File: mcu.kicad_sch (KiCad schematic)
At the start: 33 parts, among them J1 U.FL-R-SMT-1(10), U1 SF32LB525UC6, U2 MKDV1GCL-ABF, Y1 48MHz, Y2 32.768khz

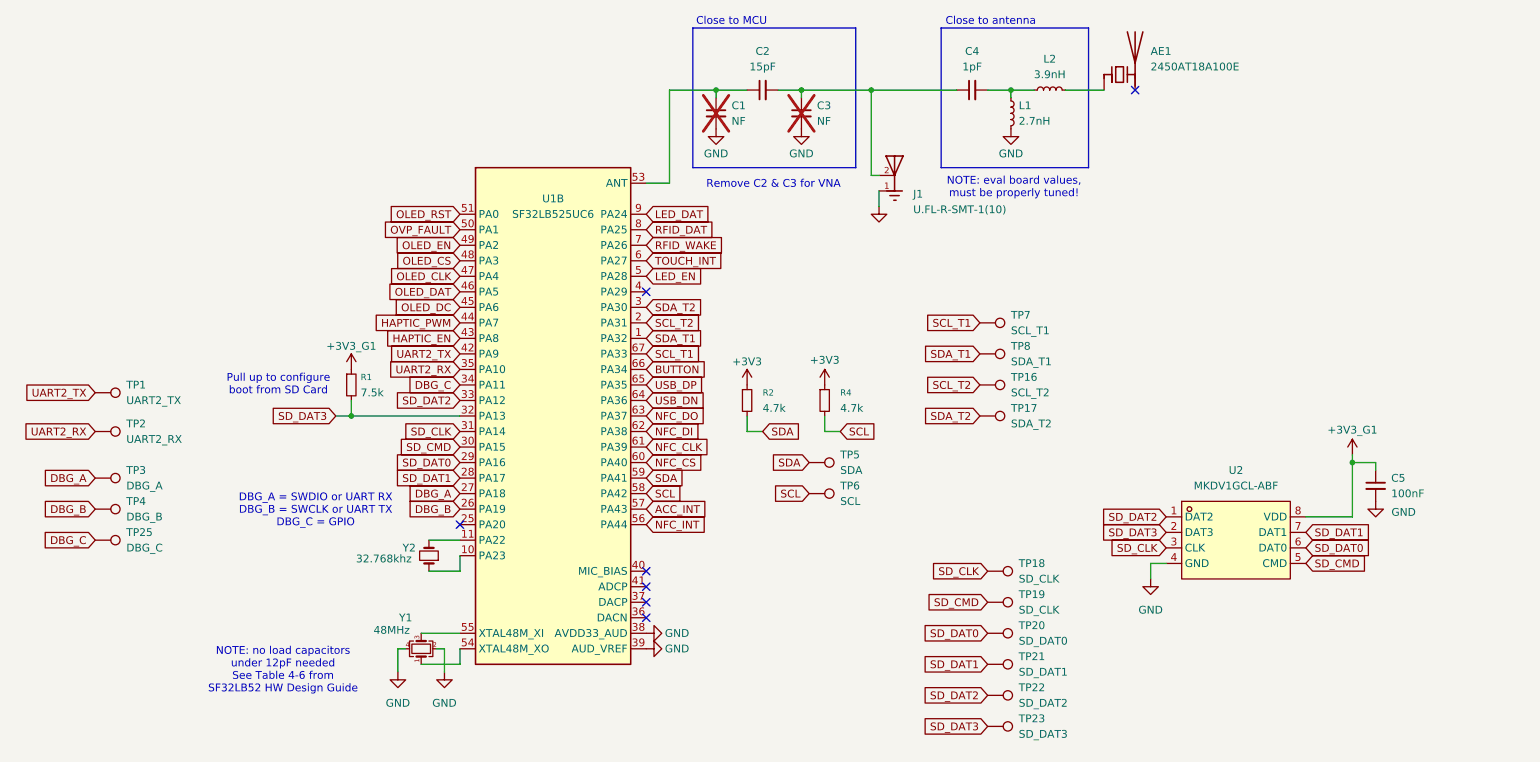
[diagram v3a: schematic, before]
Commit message: fixups before manufacturing pt2
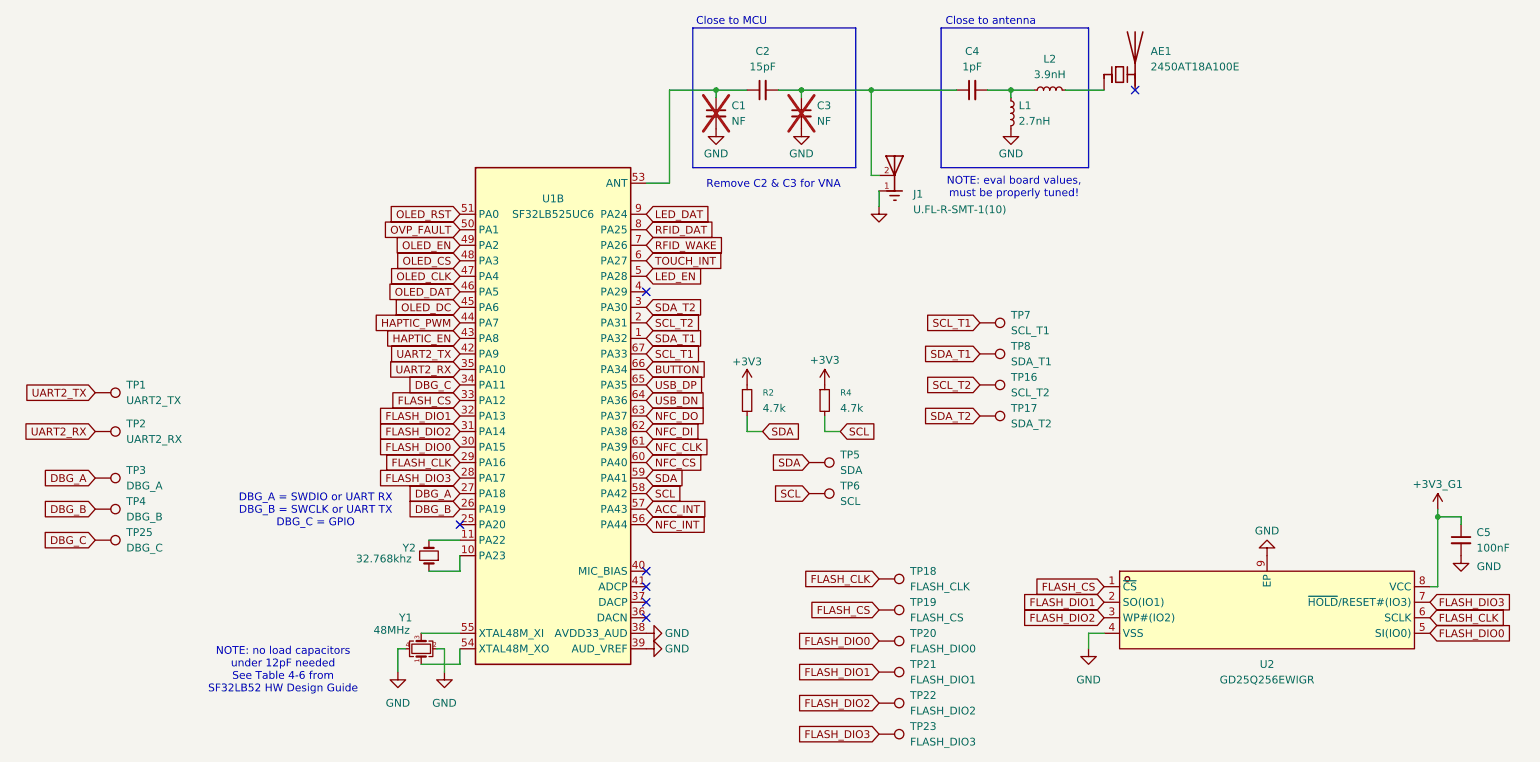
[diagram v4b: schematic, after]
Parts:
- removed R1: 7.5k, Resistor_SMD:R_0603_1608Metric, symbol Device:R_Small
- removed U2: MKDV1GCL-ABF, MKDV1GCL-ABA:LGA-8_L6.0-W8.0-P1.27-TL, symbol MKDV1GCL-ABA:MKDV1GCL-ABA
- added U2: GD25Q256EWIGR, GD25Q256EWIGR:WSON-8_L6.0-W5.0-P1.27-TL-EP, symbol GD25Q256EWIGR:GD25Q256EWIGR
- TP18: value SD_CLK -> FLASH_CLK
- TP19: value SD_CLK -> FLASH_CS
- TP20: value SD_DAT0 -> FLASH_DIO0
- TP21: value SD_DAT1 -> FLASH_DIO1
- TP22: value SD_DAT2 -> FLASH_DIO2
- TP23: value SD_DAT3 -> FLASH_DIO3
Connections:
- net +3V3_G1: now also U2.8 (VCC)
- net GND: now also U2.4 (VSS), U2.9 (EP)
- net SD_CLK renamed FLASH_CLK
- net FLASH_CLK: now also U1.29 (PA16), U2.6 (SCLK); no longer U1.31 (PA14)
- net SD_CMD renamed FLASH_CS
- net FLASH_CS: now also U1.33 (PA12), U2.1 (~{CS}); no longer U1.30 (PA15)
- net SD_DAT0 renamed FLASH_DIO0
- net FLASH_DIO0: now also U1.30 (PA15), U2.5 (SI(IO0)); no longer U1.29 (PA16)
- net SD_DAT1 renamed FLASH_DIO1
- net FLASH_DIO1: now also U1.32 (PA13), U2.2 (SO(IO1)); no longer U1.28 (PA17)
- net SD_DAT2 renamed FLASH_DIO2
- net FLASH_DIO2: now also U1.31 (PA14), U2.3 (WP#(IO2)); no longer U1.33 (PA12)
- net SD_DAT3 renamed FLASH_DIO3
- net FLASH_DIO3: now also U1.28 (PA17), U2.7 (~{HOLD}/RESET#(IO3)); no longer U1.32 (PA13)
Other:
- note removed: "Pull up to configure boot from SD Card"
- moved on the sheet: C5, TP18, TP19, TP20, TP21, TP22, TP23

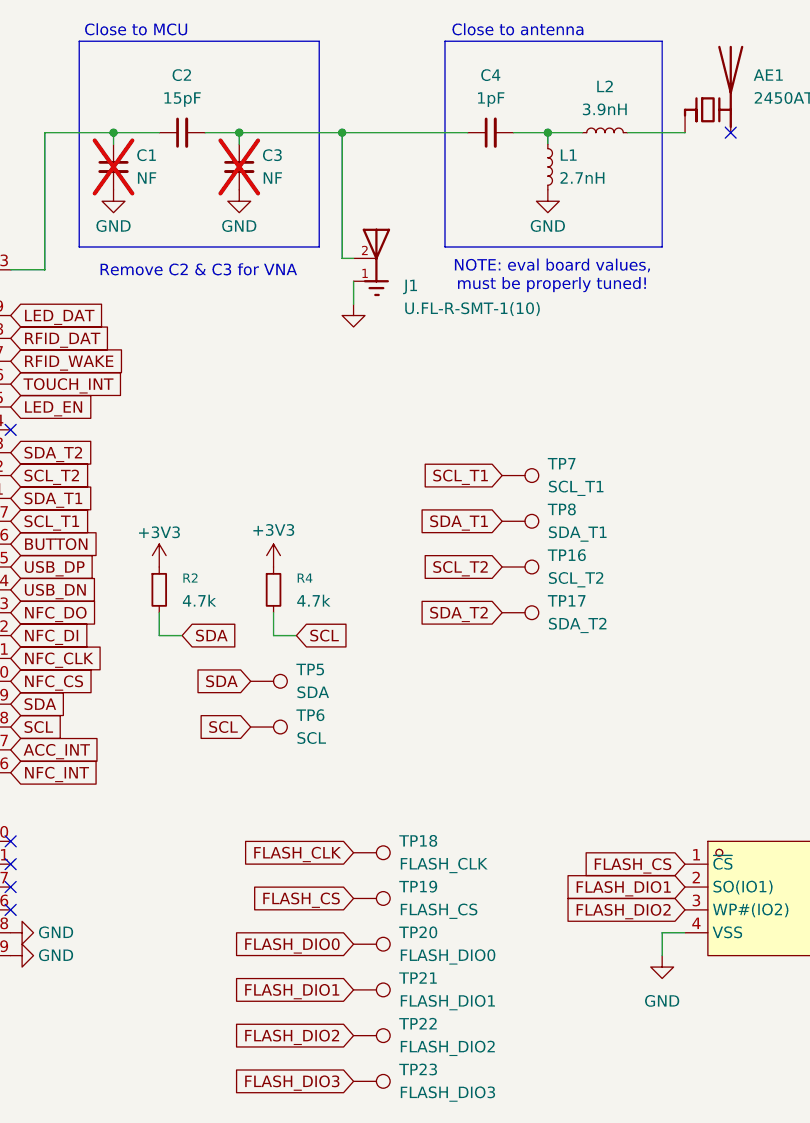
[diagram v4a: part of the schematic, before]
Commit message: layout progress
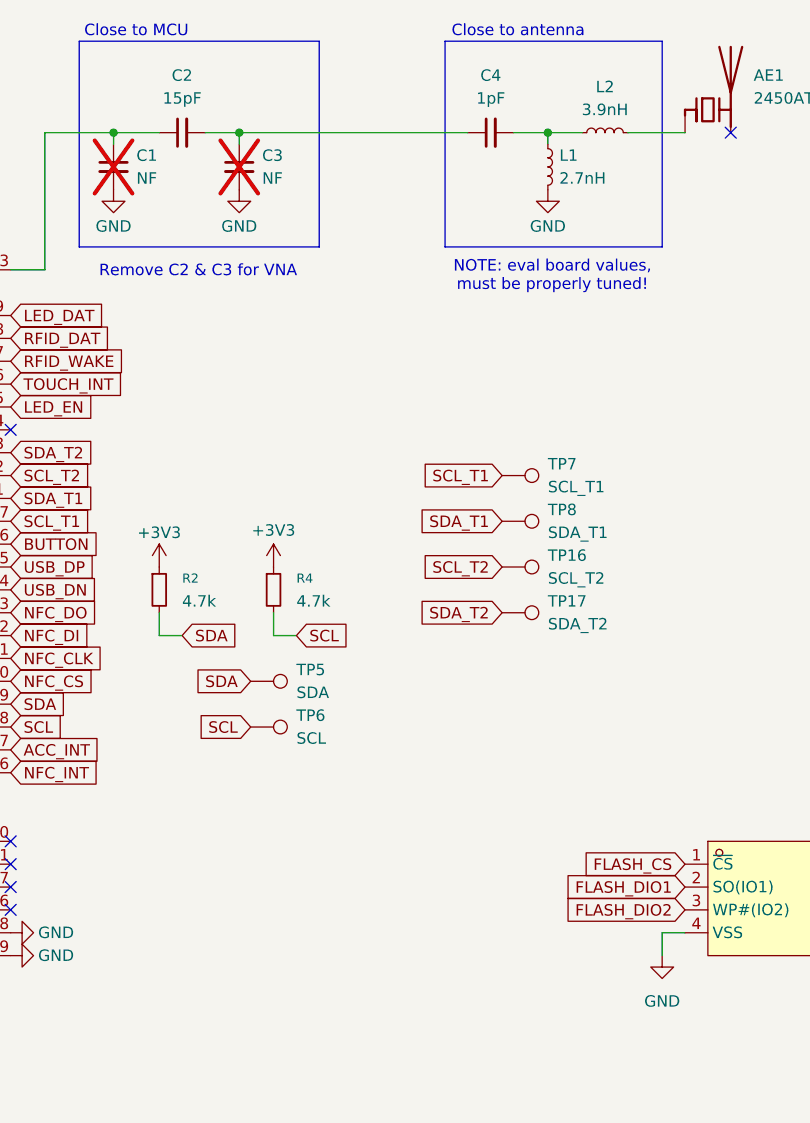
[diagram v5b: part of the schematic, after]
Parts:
- removed J1: U.FL-R-SMT-1(10), U.FL-R-SMT-1_10_:HRS_U.FL-R-SMT-1_10_, symbol U.FL-R-SMT-1_10_:U.FL-R-SMT-1_10_
- removed TP18: FLASH_CLK, TestPoint:TestPoint_Pad_D1.0mm, symbol Connector:TestPoint
- removed TP19: FLASH_CS, TestPoint:TestPoint_Pad_D1.0mm, symbol Connector:TestPoint
- removed TP20: FLASH_DIO0, TestPoint:TestPoint_Pad_D1.0mm, symbol Connector:TestPoint
- removed TP21: FLASH_DIO1, TestPoint:TestPoint_Pad_D1.0mm, symbol Connector:TestPoint
- removed TP22: FLASH_DIO2, TestPoint:TestPoint_Pad_D1.0mm, symbol Connector:TestPoint
- removed TP23: FLASH_DIO3, TestPoint:TestPoint_Pad_D1.0mm, symbol Connector:TestPoint

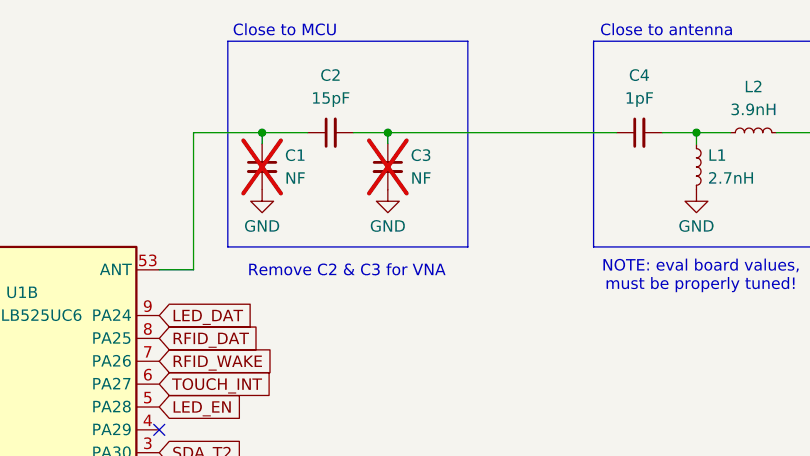
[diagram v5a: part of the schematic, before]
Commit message: progress
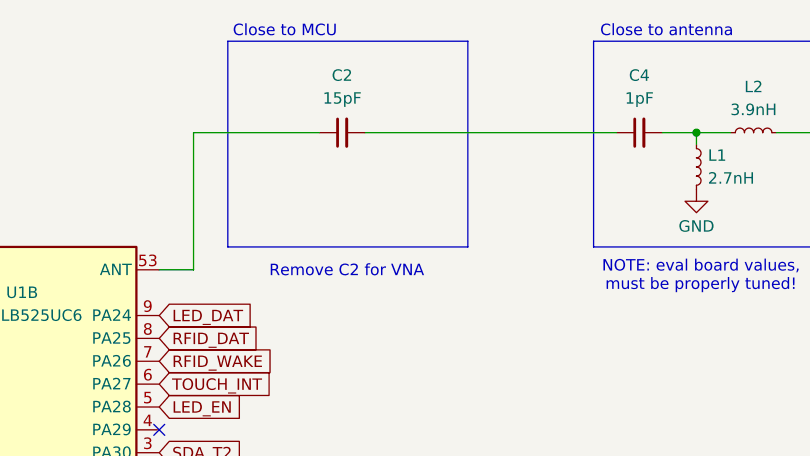
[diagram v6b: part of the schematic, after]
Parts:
- removed C1, C3: NF, Capacitor_SMD:C_0402_1005Metric, symbol Device:C_Small
- Y1: footprint Crystal:Crystal_SMD_2520-4Pin_2.5x2.0mm -> Crystal:Crystal_SMD_2016-4Pin_2.0x1.6mm; LCSC Part C2932991 -> C49363531
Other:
- note added: "Remove C2 for VNA"
- note removed: "Remove C2 & C3 for VNA"
- moved on the sheet: C2

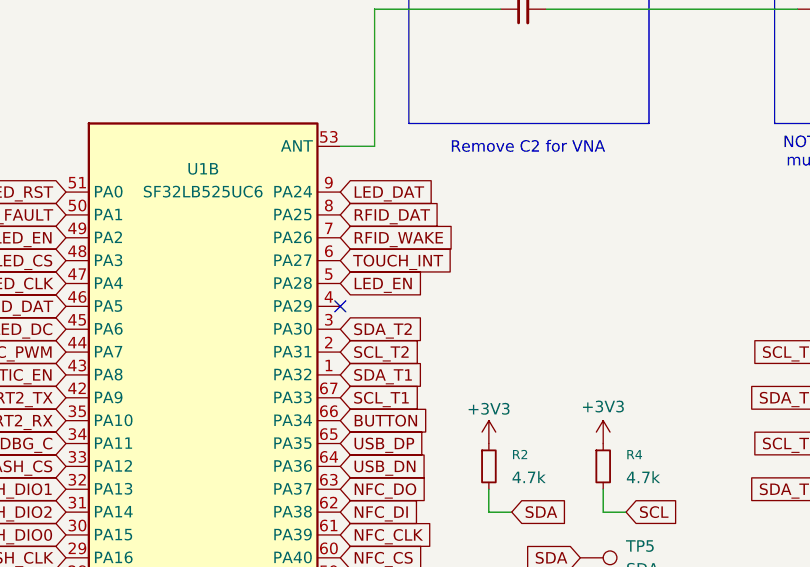
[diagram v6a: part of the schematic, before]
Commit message: progress before restarting bigtime
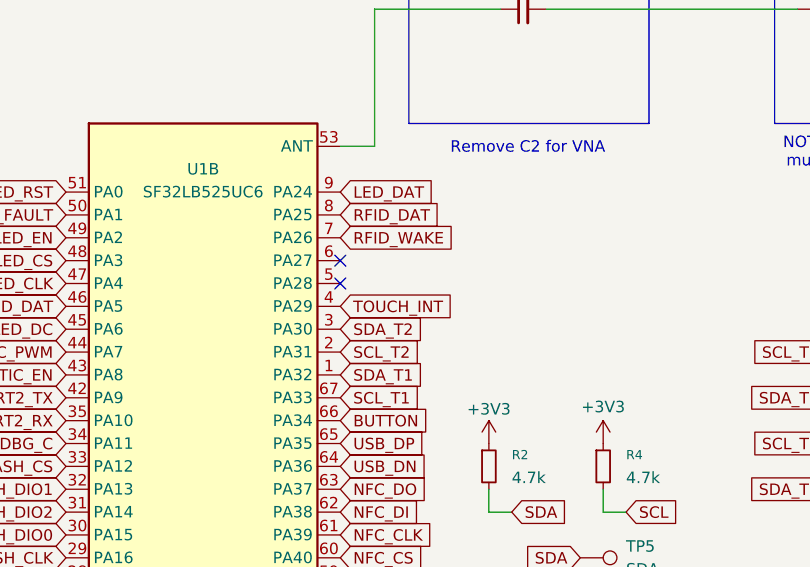
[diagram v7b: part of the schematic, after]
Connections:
- net TOUCH_INT: now also U1.4 (PA29); no longer U1.6 (PA27)
- net LED_EN: no longer names the net of U1.5 (PA28)
- no-connect marks 7 -> 8
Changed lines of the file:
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@@
+	)
+	(no_connect
+		(at 137.16 78.74)
+	)
+	(no_connect
+		(at 137.16 81.28)
 	)
 	(no_connect
@@
 	)
 	(no_connect
-		(at 137.16 83.82)
-	)
-	(no_connect
 		(at 137.16 129.54)
 	)
@@
 	(global_label "TOUCH_INT"
 		(shape input)
-		(at 137.16 78.74 0)
+		(at 137.16 83.82 0)
 		(fields_autoplaced yes)
 		(effects
@@
 		)
 		(property "Intersheetrefs" "${INTERSHEET_REFS}"
-			(at 150.2448 78.74 0)
+			(at 150.2448 83.82 0)
 			(effects
 				(font
@@
 			(effects
 				(font
-					(size 1.27 1.27)
-				)
-				(justify left)
-				(hide yes)
-			)
-		)
-	)
-	(global_label "LED_EN"
-		(shape input)
-		(at 137.16 81.28 0)
-		(fields_autoplaced yes)
-		(effects
-			(font
-				(size 1.27 1.27)
-			)
-			(justify left)
-		)
-		(property "Intersheetrefs" "${INTERSHEET_REFS}"
-			(at 147.0394 81.28 0)
-			(effects
-				(font

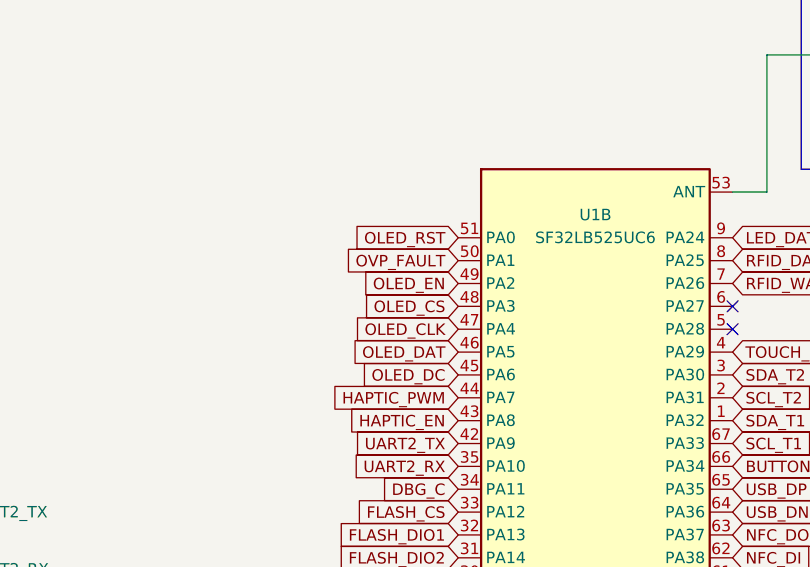
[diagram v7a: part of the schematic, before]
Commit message: huge progress
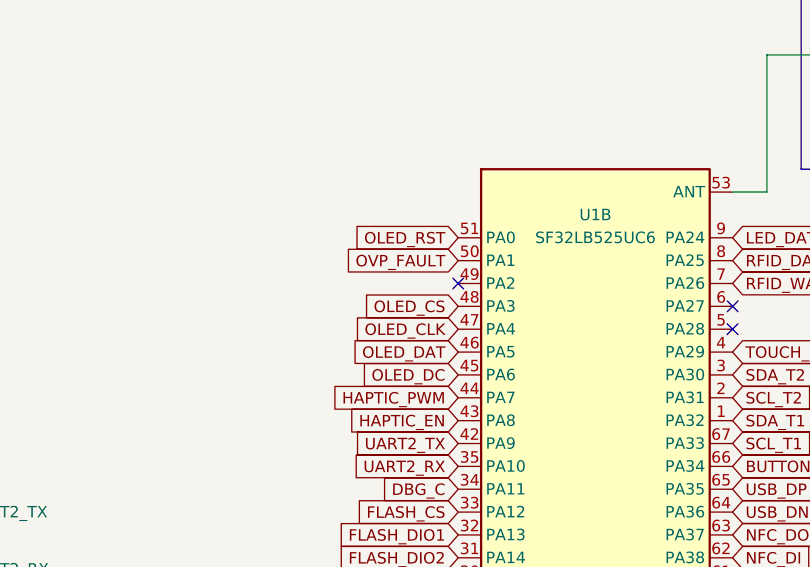
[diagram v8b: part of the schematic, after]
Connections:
- net OLED_EN: no longer names the net of U1.49 (PA2)
- no-connect marks 8 -> 9
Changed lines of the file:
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@@
+	)
+	(no_connect
+		(at 106.68 76.2)
 	)
 	(no_connect
@@
 			(effects
 				(font
-					(size 1.27 1.27)
-				)
-				(justify right)
-				(hide yes)
-			)
-		)
-	)
-	(global_label "OLED_EN"
-		(shape input)
-		(at 106.68 76.2 180)
-		(fields_autoplaced yes)
-		(effects
-			(font
-				(size 1.27 1.27)
-			)
-			(justify right)
-		)
-		(property "Intersheetrefs" "${INTERSHEET_REFS}"
-			(at 95.4701 76.2 0)
-			(effects
-				(font
